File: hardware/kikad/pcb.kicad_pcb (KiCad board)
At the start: 2 copper layers, 45 x 45 mm, 21 parts, among them J2 BOARD

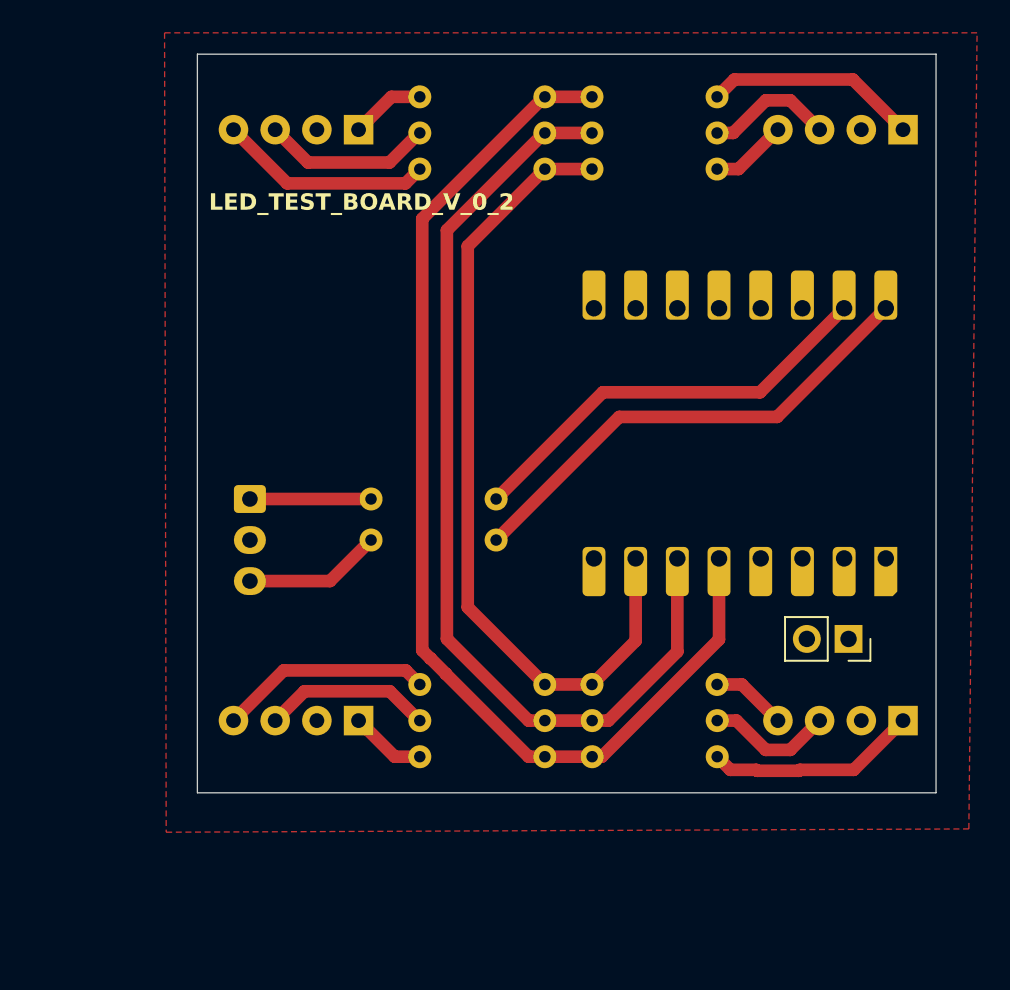
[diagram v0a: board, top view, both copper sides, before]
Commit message: make the v0.3 read to use
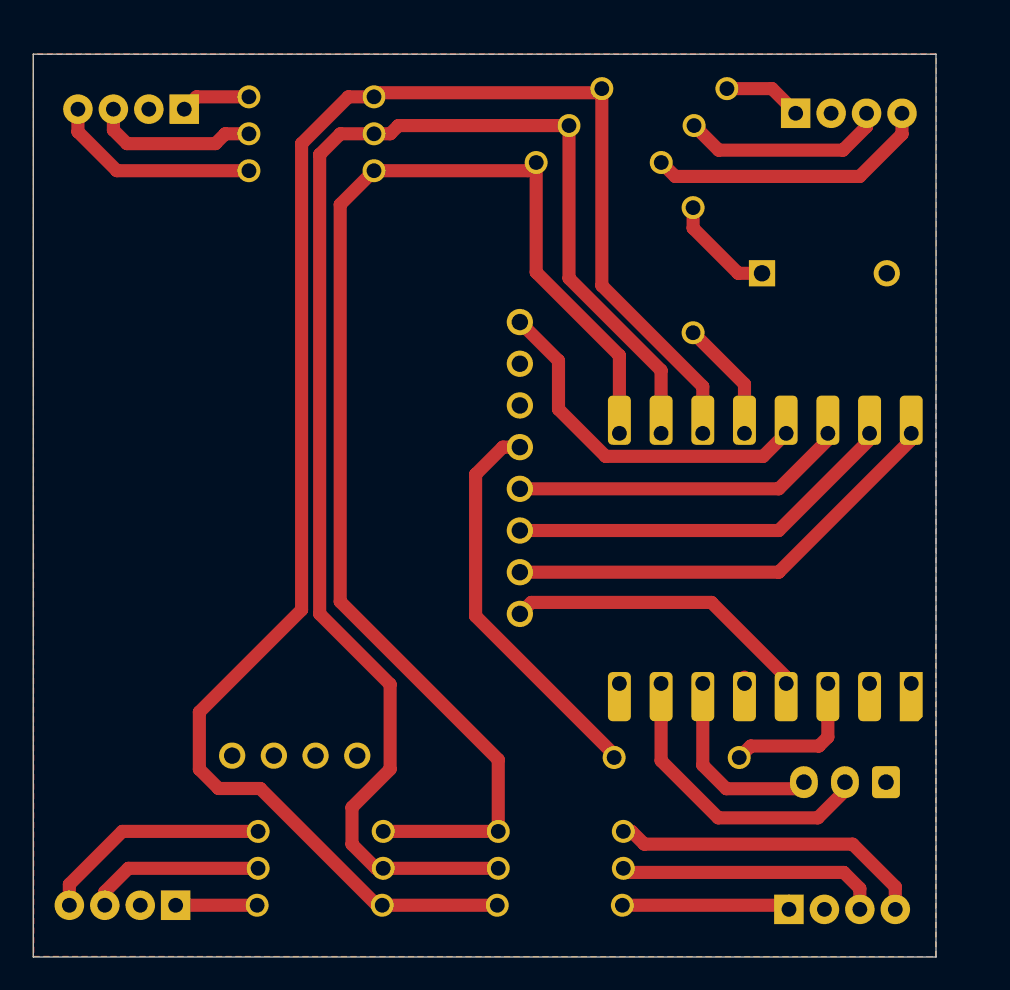
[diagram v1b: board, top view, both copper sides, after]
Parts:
- removed D7: LED_Dual_AKA, Connector_JST:JST_XH_B3B-XH-A_1x03_P2.50mm_Vertical
- removed J2: BOARD, Connector_PinSocket_2.54mm:PinSocket_1x02_P2.54mm_Vertical
- added BZ1: Buzzer, Buzzer_Beeper:MagneticBuzzer_ProSignal_ABI-010-RC, B.Cu at (144.4, 53.4)
- added J1: Output, Connector_JST:JST_XH_B3B-XH-A_1x03_P2.50mm_Vertical, B.Cu at (151.9, 84.3)
- added U2: ~, esp_32_c3_supper_mini:PN532 NFC RFID, B.Cu at (117.2, 67.5)
- D1, D2, D3, D4: footprint LED_THT:LED_D5.0mm-4_RGB_Wide_Pins_custom -> LED_THT:LED_D5.0mm-4_RGB_Wide_Pins
- R14: value 150 -> 0
- moved R13 22.1 mm to (140.2, 57.0), turned to 90 degrees
- moved D4 15.8 mm to (108.7, 91.8)
- moved R14 15.1 mm to (135.4, 82.8), turned to 0 degrees
- moved D3 13.4 mm to (146.0, 92.1), turned to 0 degrees
- moved R12 13.4 mm to (121.3, 91.8)
- moved R11 13.3 mm to (121.3, 89.6)
- moved R10 13.3 mm to (121.3, 87.3)
- moved R9 10.7 mm to (128.3, 91.8)
- moved D2 10.7 mm to (109.2, 43.4)
- moved R8 10.7 mm to (128.3, 89.6)
- moved R7 10.6 mm to (128.3, 87.3)
- moved R4 10.4 mm to (120.8, 47.1)
- moved R5 10.4 mm to (120.8, 44.9)
- moved R6 10.4 mm to (120.8, 42.6)
- moved U1 7.78 mm to (143.5, 70.7)
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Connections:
- R13 pad 1: Net-(D7-A1) -> Net-(U1-GPIO9/SCL)
- R13 pad 2: Net-(U1-GPIO6) -> Net-(BZ1-+)
- R14 pad 1: Net-(U1-GPIO5) -> Net-(R14-Pad1)
- R14 pad 2: Net-(D7-A2) -> Net-(U1-3V3)
- U1 pad 1: (no net) -> unconnected-(U1-5V-Pad1)
- U1 pad 10: Net-(U1-GPIO6) -> Net-(U1-GPIO6/MOSI)
- U1 pad 11: unconnected-(U1-GPIO7-Pad11) -> Net-(U1-GPIO7/SS)
- U1 pad 12: unconnected-(U1-GPIO8-Pad12) -> Net-(U1-GPIO8/SDA)
- U1 pad 13: unconnected-(U1-GPIO9-Pad13) -> Net-(U1-GPIO9/SCL)
- U1 pad 14: unconnected-(U1-GPIO10-Pad14) -> /R
- U1 pad 15: unconnected-(U1-GPIO20-Pad15) -> /G
- U1 pad 16: unconnected-(U1-GPIO21-Pad16) -> /B
- U1 pad 3: unconnected-(U1-3V3-Pad3) -> Net-(U1-3V3)
- U1 pad 4: unconnected-(U1-GPIO4-Pad4) -> Net-(U1-GPIO4/SCK)
- U1 pad 5: /R -> unconnected-(U1-GPIO3-Pad5)
- U1 pad 6: /G -> Net-(J1-Pin_3)
- U1 pad 7: /B -> Net-(J1-Pin_2)
- U1 pad 9: Net-(U1-GPIO5) -> Net-(U1-GPIO5/MISO)
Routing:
- net /R: track 68.4 -> 105.5 mm
- net /G: track 59.7 -> 91.3 mm
- net /B: track 49.8 -> 80.8 mm
- net Net-(U1-GPIO5): track 29.6 -> 0.00 mm
- net Net-(U1-GPIO5/MISO): track 0.00 -> 27.6 mm
- net Net-(U1-GPIO6): track 26.0 -> 0.00 mm
- net Net-(R14-Pad1): track 0.00 -> 24.4 mm
- net Net-(U1-GPIO6/MOSI): track 0.00 -> 24.0 mm
- net Net-(U1-GPIO8/SDA): track 0.00 -> 21.9 mm
- net Net-(U1-GPIO7/SS): track 0.00 -> 20.4 mm
- net Net-(U1-GPIO4/SCK): track 0.00 -> 18.8 mm
- net Net-(J1-Pin_2): track 0.00 -> 18.6 mm
- net Net-(D3-BA): track 4.62 -> 19.3 mm
- net Net-(D1-BA): track 4.70 -> 17.4 mm
- net Net-(J1-Pin_3): track 0.00 -> 11.9 mm
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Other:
- board size 45 x 45 mm -> 55 x 55 mm
- board text removed: "LED_TEST_BOARD_V_0_2"

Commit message: Revert "make the v0.3 read to use"
This reverts commit 2651ca28fcff3cfeeb4fb146a67662ef7f719936.
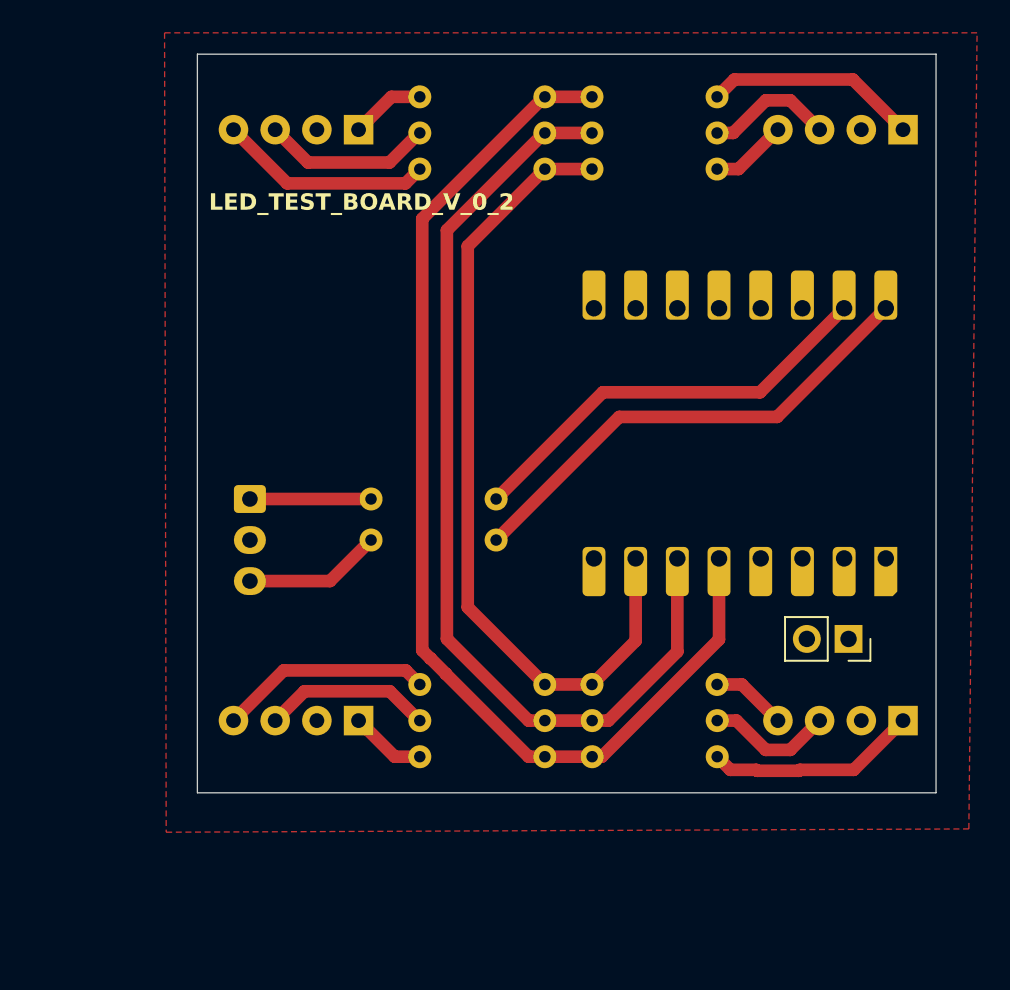
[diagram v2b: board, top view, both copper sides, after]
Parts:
- removed BZ1: Buzzer, Buzzer_Beeper:MagneticBuzzer_ProSignal_ABI-010-RC
- removed J1: Output, Connector_JST:JST_XH_B3B-XH-A_1x03_P2.50mm_Vertical
- removed U2: ~, esp_32_c3_supper_mini:PN532 NFC RFID
- added D7: LED_Dual_AKA, Connector_JST:JST_XH_B3B-XH-A_1x03_P2.50mm_Vertical, B.Cu at (113.2, 67.1)
- added J2: BOARD, Connector_PinSocket_2.54mm:PinSocket_1x02_P2.54mm_Vertical, F.Cu at (149.7, 75.6)
- D1, D2, D3, D4: footprint LED_THT:LED_D5.0mm-4_RGB_Wide_Pins -> LED_THT:LED_D5.0mm-4_RGB_Wide_Pins_custom
- R14: value 0 -> 150
- moved R13 22.1 mm to (120.6, 67.1), turned to 0 degrees
- moved D4 15.8 mm to (119.8, 80.6)
- moved R14 15.1 mm to (128.2, 69.6), turned to 180 degrees
- moved D3 13.4 mm to (153.0, 80.6), turned to 180 degrees
- moved R12 13.4 mm to (131.2, 82.8)
- moved R11 13.3 mm to (131.2, 80.6)
- moved R10 13.3 mm to (131.2, 78.4)
- moved R9 10.7 mm to (134.1, 82.8)
- moved D2 10.7 mm to (119.8, 44.6)
- moved R8 10.7 mm to (134.1, 80.6)
- moved R7 10.6 mm to (134.0, 78.4)
- moved R4 10.4 mm to (131.2, 47.0)
- moved R5 10.4 mm to (131.2, 44.8)
- moved R6 10.4 mm to (131.2, 42.6)
- moved U1 7.78 mm to (141.9, 63.1)
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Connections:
- R13 pad 1: Net-(U1-GPIO9/SCL) -> Net-(D7-A1)
- R13 pad 2: Net-(BZ1-+) -> Net-(U1-GPIO6)
- R14 pad 1: Net-(R14-Pad1) -> Net-(U1-GPIO5)
- R14 pad 2: Net-(U1-3V3) -> Net-(D7-A2)
- U1 pad 1: unconnected-(U1-5V-Pad1) -> (no net)
- U1 pad 10: Net-(U1-GPIO6/MOSI) -> Net-(U1-GPIO6)
- U1 pad 11: Net-(U1-GPIO7/SS) -> unconnected-(U1-GPIO7-Pad11)
- U1 pad 12: Net-(U1-GPIO8/SDA) -> unconnected-(U1-GPIO8-Pad12)
- U1 pad 13: Net-(U1-GPIO9/SCL) -> unconnected-(U1-GPIO9-Pad13)
- U1 pad 14: /R -> unconnected-(U1-GPIO10-Pad14)
- U1 pad 15: /G -> unconnected-(U1-GPIO20-Pad15)
- U1 pad 16: /B -> unconnected-(U1-GPIO21-Pad16)
- U1 pad 3: Net-(U1-3V3) -> unconnected-(U1-3V3-Pad3)
- U1 pad 4: Net-(U1-GPIO4/SCK) -> unconnected-(U1-GPIO4-Pad4)
- U1 pad 5: unconnected-(U1-GPIO3-Pad5) -> /R
- U1 pad 6: Net-(J1-Pin_3) -> /G
- U1 pad 7: Net-(J1-Pin_2) -> /B
- U1 pad 9: Net-(U1-GPIO5/MISO) -> Net-(U1-GPIO5)
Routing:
- net /R: track 105.5 -> 68.4 mm
- net /G: track 91.3 -> 59.7 mm
- net /B: track 80.8 -> 49.8 mm
- net Net-(U1-GPIO5): track 0.00 -> 29.6 mm
- net Net-(U1-GPIO5/MISO): track 27.6 -> 0.00 mm
- net Net-(U1-GPIO6): track 0.00 -> 26.0 mm
- net Net-(R14-Pad1): track 24.4 -> 0.00 mm
- net Net-(U1-GPIO6/MOSI): track 24.0 -> 0.00 mm
- net Net-(U1-GPIO8/SDA): track 21.9 -> 0.00 mm
- net Net-(U1-GPIO7/SS): track 20.4 -> 0.00 mm
- net Net-(U1-GPIO4/SCK): track 18.8 -> 0.00 mm
- net Net-(J1-Pin_2): track 18.6 -> 0.00 mm
- net Net-(D3-BA): track 19.3 -> 4.62 mm
- net Net-(D1-BA): track 17.4 -> 4.70 mm
- net Net-(J1-Pin_3): track 11.9 -> 0.00 mm
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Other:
- board size 55 x 55 mm -> 45 x 45 mm
- board text added: "LED_TEST_BOARD_V_0_2"
